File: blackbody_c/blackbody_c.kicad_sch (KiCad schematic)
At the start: 3 parts, among them J1 Conn_01x04_Pin, J2 Conn_01x04_Pin

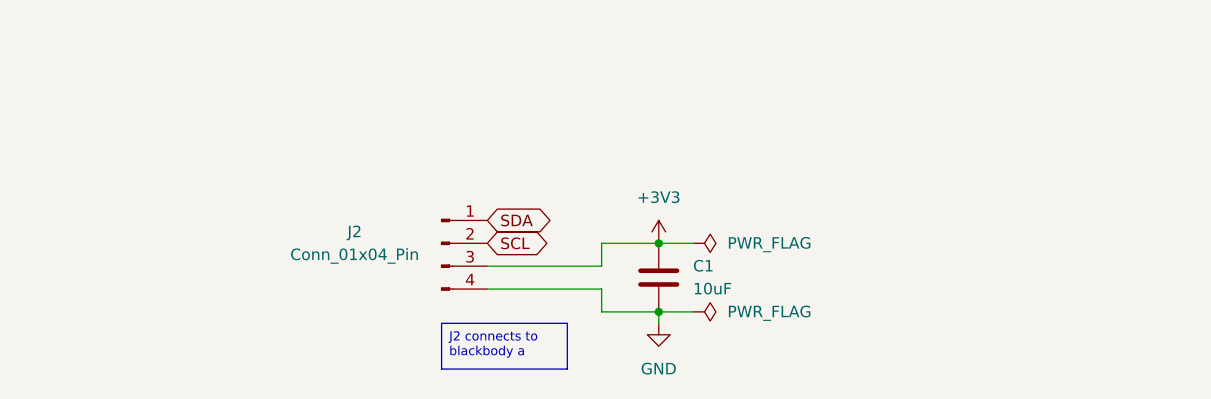
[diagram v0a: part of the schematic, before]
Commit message: Updated minor errors
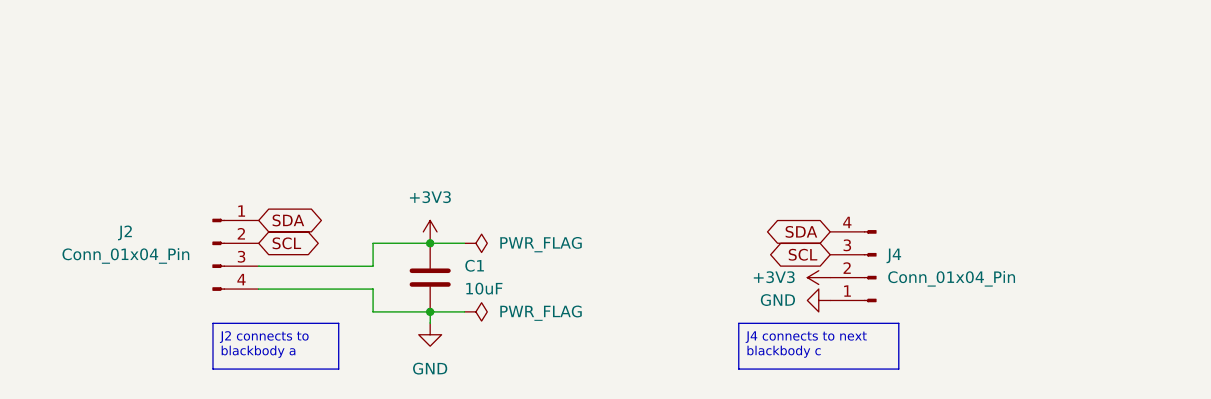
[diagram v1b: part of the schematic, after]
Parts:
- added J4: Conn_01x04_Pin, symbol Connector:Conn_01x04_Pin
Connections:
- net +3V3: now also J4.2 (Pin_2)
- net GND: now also J4.1 (Pin_1)
- net SCL: now also J4.3 (Pin_3)
- net SDA: now also J4.4 (Pin_4)
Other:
- moved on the sheet: C1, J2

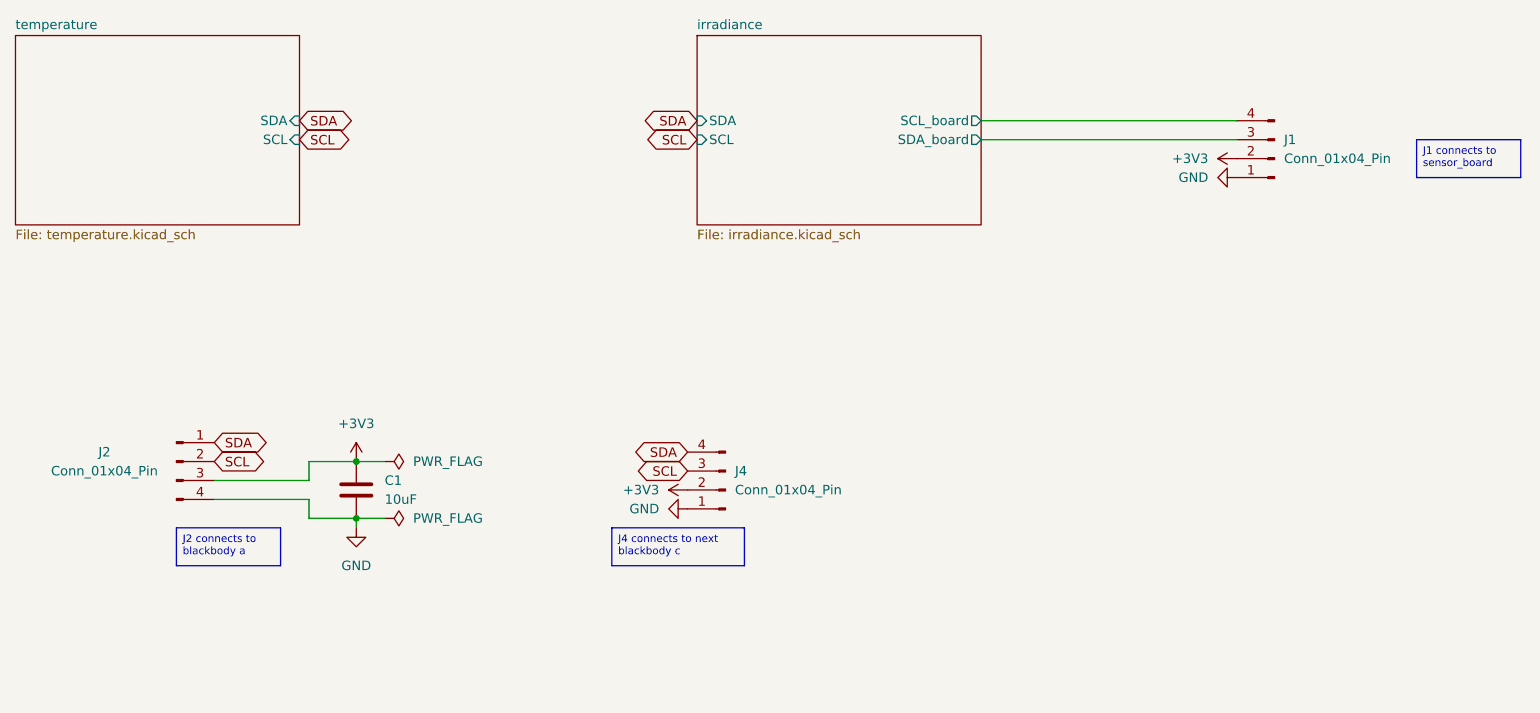
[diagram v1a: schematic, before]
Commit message: Fixed pins, minor changes, removed power isolation
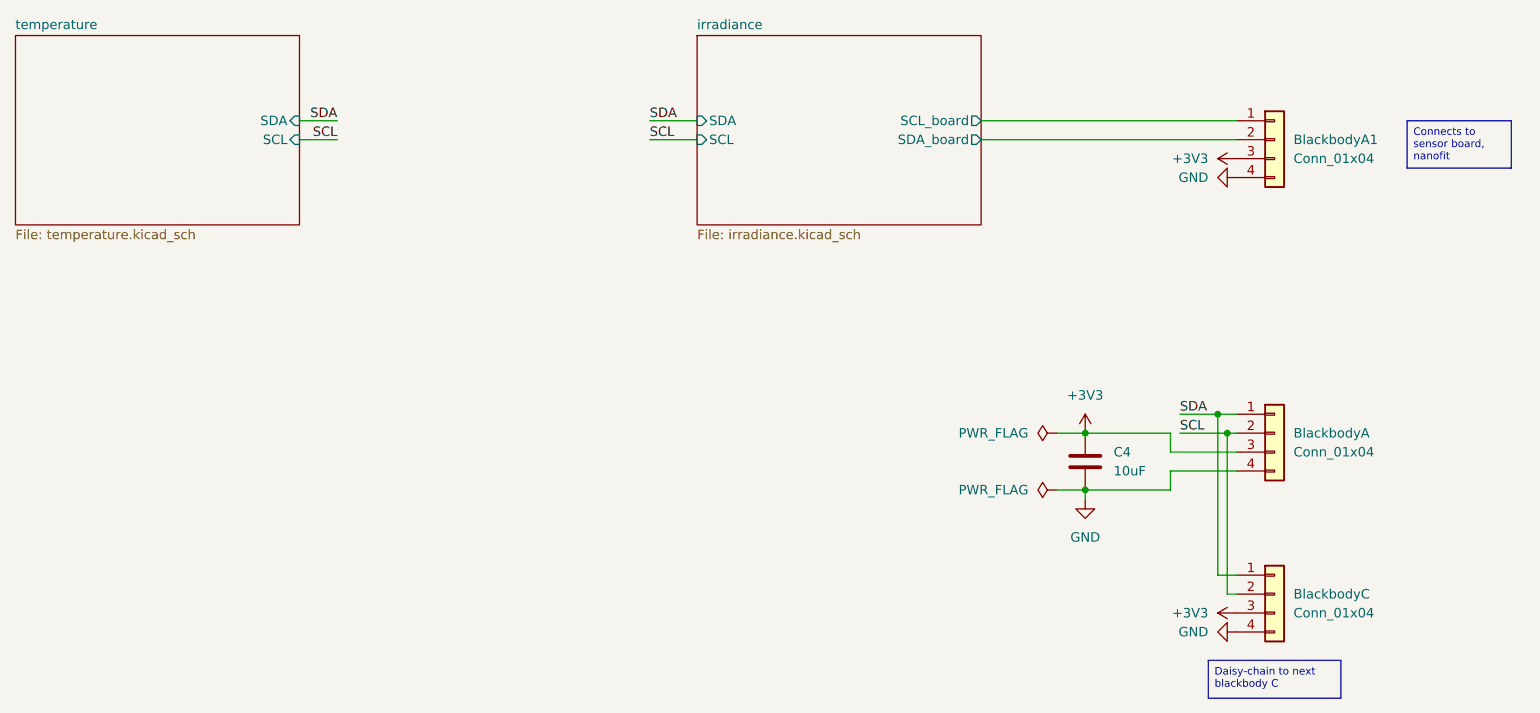
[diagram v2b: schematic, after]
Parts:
- removed C1: 10uF, symbol Device:C
- removed J1, J2, J4: Conn_01x04_Pin, symbol Connector:Conn_01x04_Pin
- added BlackbodyA, BlackbodyA1, BlackbodyC: Conn_01x04, symbol Connector_Generic:Conn_01x04
- added C4: 10uF, symbol Device:C
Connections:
- net +3V3: now also BlackbodyA.3 (Pin_3), BlackbodyA1.3 (Pin_3), BlackbodyC.3 (Pin_3), C4.1
- net GND: now also BlackbodyA.4 (Pin_4), BlackbodyA1.4 (Pin_4), BlackbodyC.4 (Pin_4), C4.2
- net SCL: now also BlackbodyA.2 (Pin_2), BlackbodyC.2 (Pin_2)
- net SDA: now also BlackbodyA.1 (Pin_1), BlackbodyC.1 (Pin_1)
- net irradiance/SCL_board: now also BlackbodyA1.1 (Pin_1)
- net irradiance/SDA_board: now also BlackbodyA1.2 (Pin_2)
